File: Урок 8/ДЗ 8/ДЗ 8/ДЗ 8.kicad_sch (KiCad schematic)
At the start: 30 parts, among them K1 HONGFA_HFD2-0xx-x-L2-x, K2 HONGFA_HFD2-0xx-x-L2-x, SW1 SW_Push, SW2 SW_Push

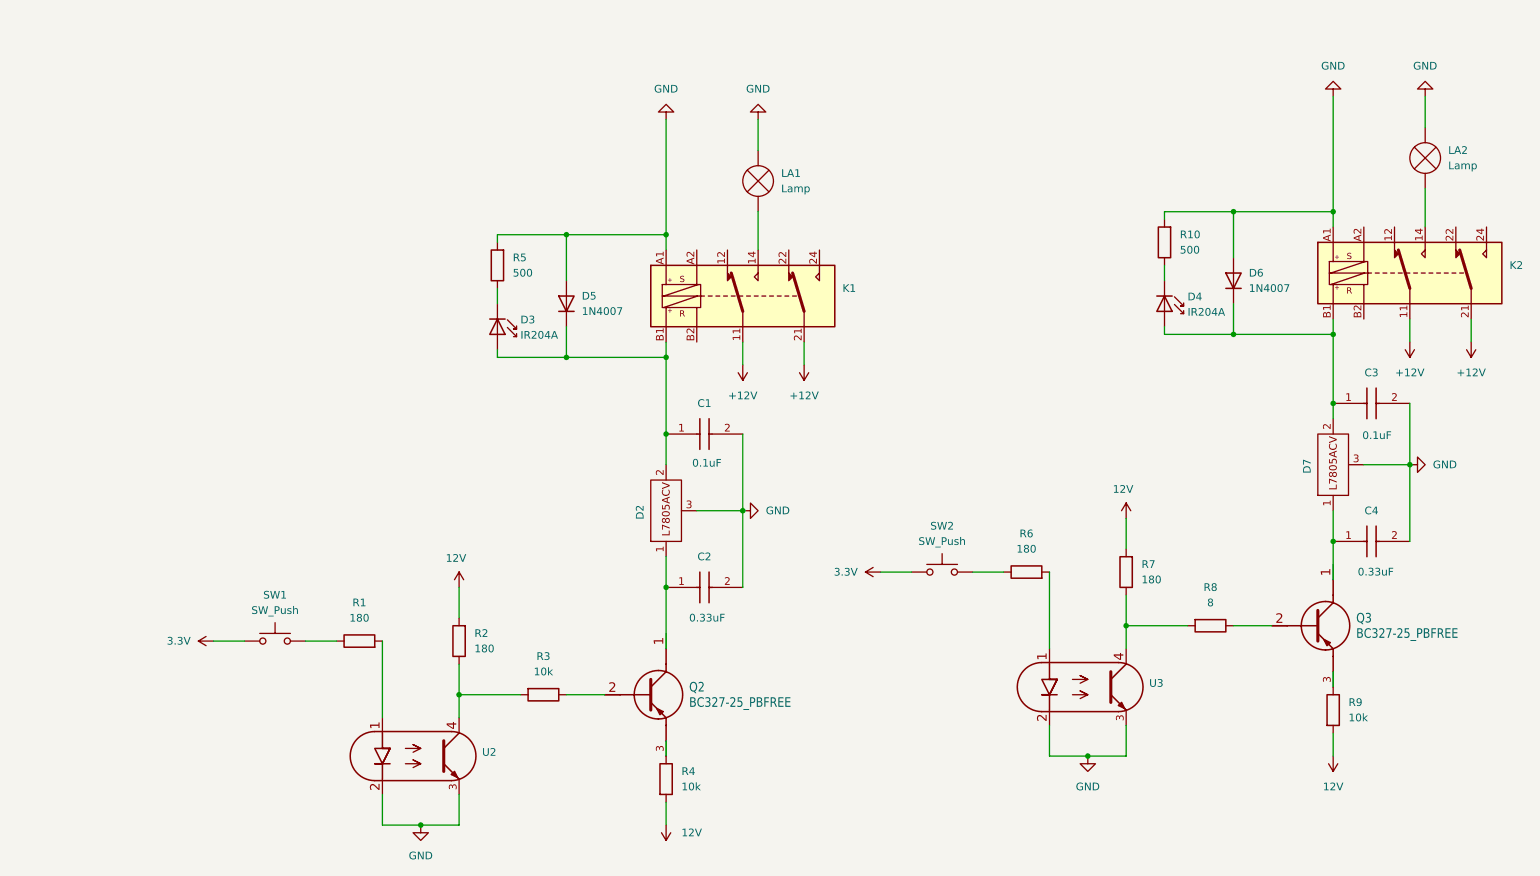
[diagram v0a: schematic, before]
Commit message: 1
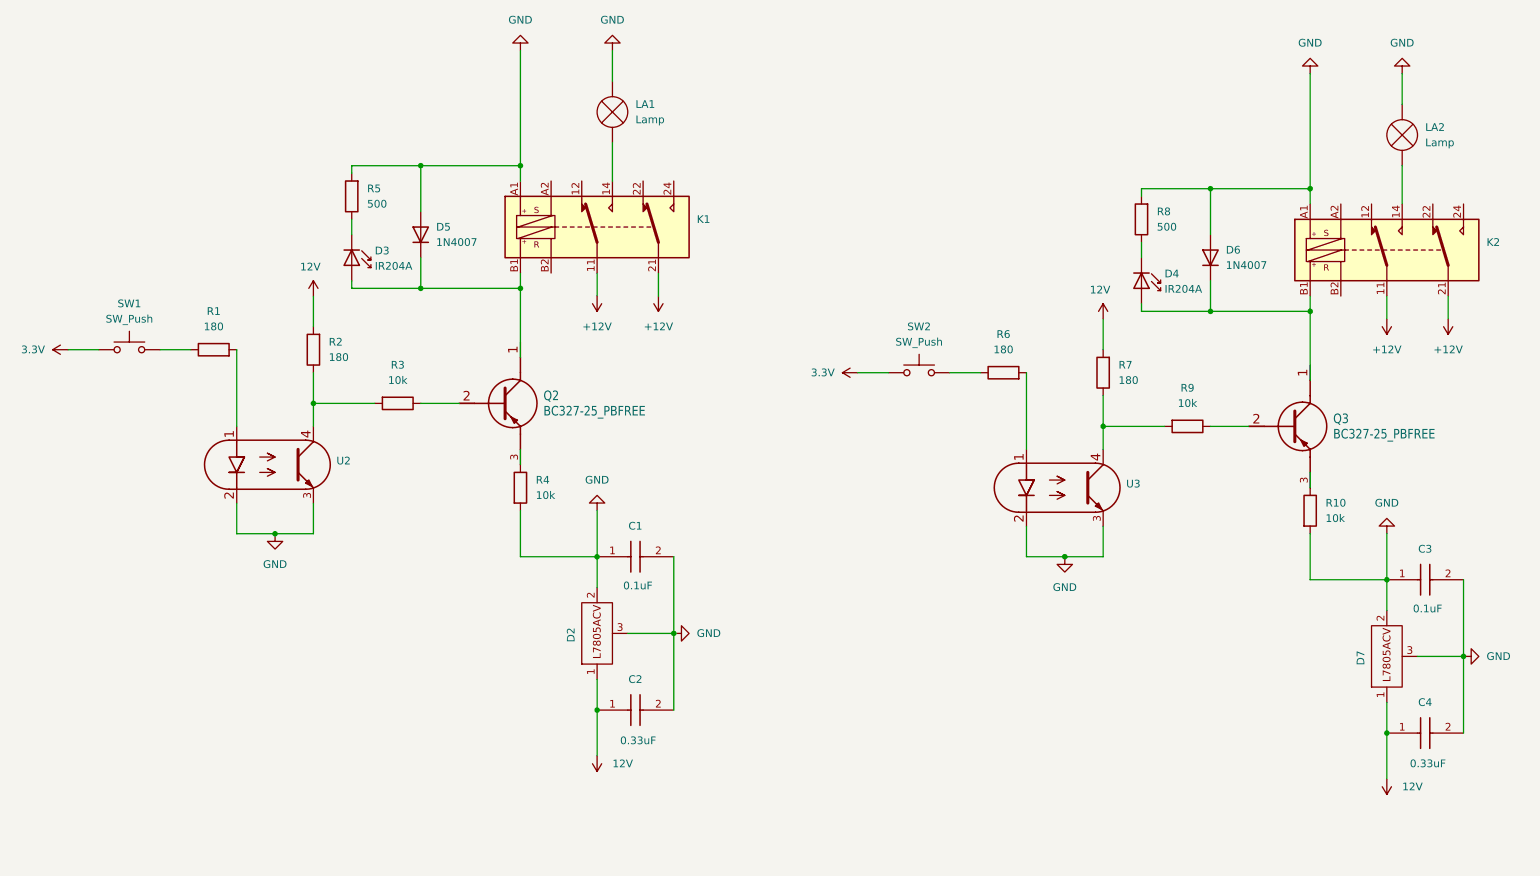
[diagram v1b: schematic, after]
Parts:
- R10: value 500 -> 10k
- R8: value 8 -> 500
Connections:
- net 12V: now also C2.1, C4.1, D2.1, D7.1; no longer R4.2, R9.2
- net GND: now also C1.1, C3.1, D2.2, D7.2, R4.2, R8.2
- net at D4.2 (A), D6.1 (K), K2.B1: now also Q3.1 (C); no longer C3.1, D7.2
- net at Q3.2 (B): now also R9.1; no longer R8.1
- net at R7.1, U3.4 (Collector): now also R9.2; no longer R8.2
- net at Q3.3 (A): now also R10.1; no longer R9.1
- net at D3.2 (A), D5.1 (K), K1.B1: now also Q2.1 (C); no longer C1.1, D2.2
- net at D4.1 (K): now also R8.1; no longer R10.1
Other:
- moved on the sheet: C1, C2, D2, D3, D5, K1, LA1, Q2, R1, R2, R3, R4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
